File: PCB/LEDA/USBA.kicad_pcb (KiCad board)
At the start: 2 copper layers, 70 x 70 mm, 23 parts, among them J1 USB_A, J2 Conn_01x03, T1 T3902_MEMS_Mic, U2 ESP32-S3-MINI-1, U5 MD8942

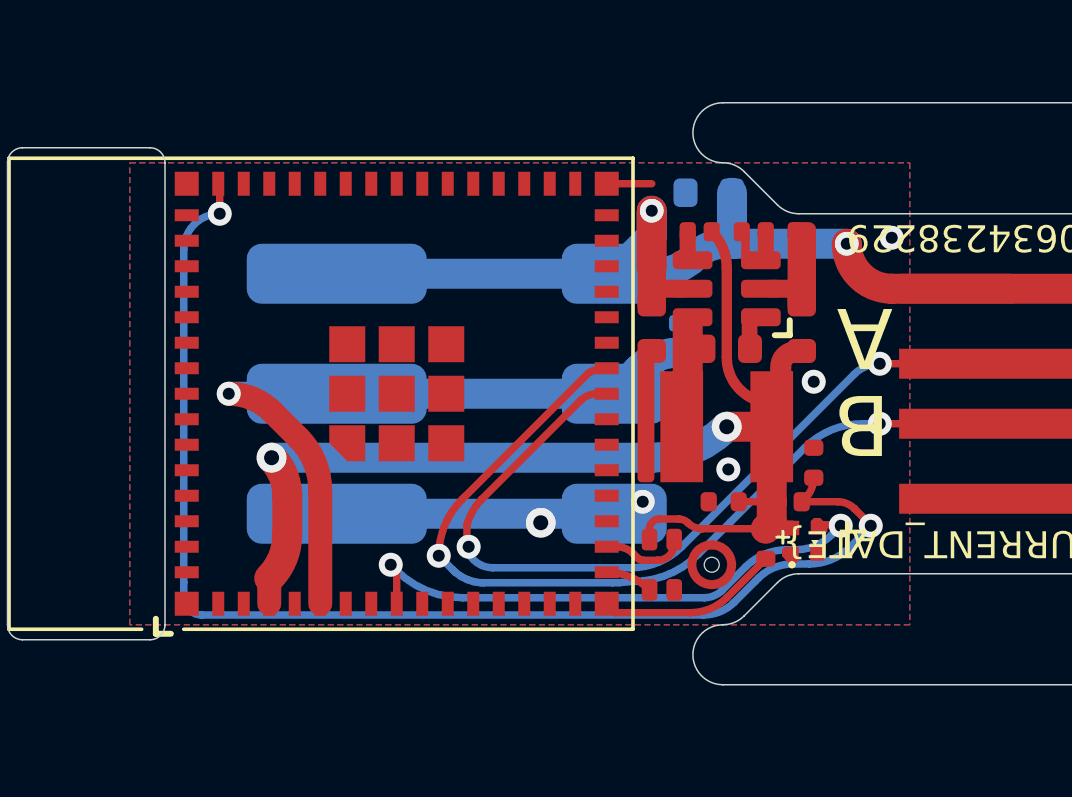
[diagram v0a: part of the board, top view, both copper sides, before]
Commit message: LEFT
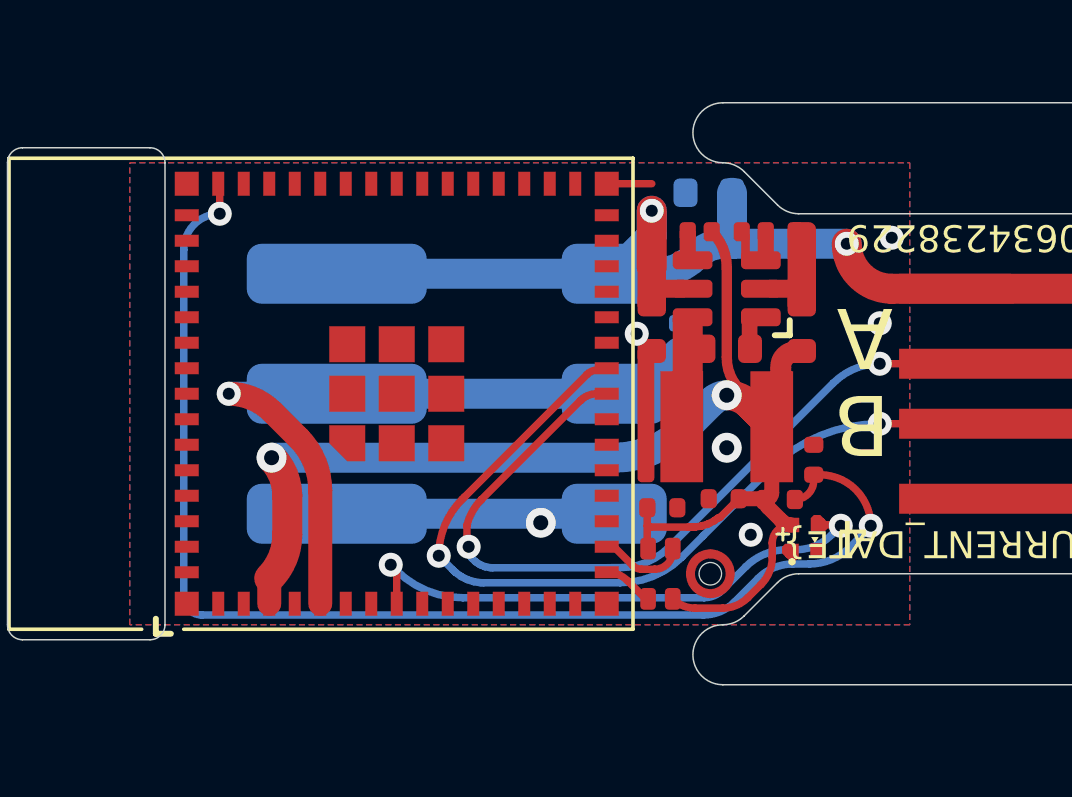
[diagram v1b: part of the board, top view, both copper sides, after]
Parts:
- moved C2 3.65 mm to (104.5, 103.1), turned to 0 degrees
- moved T1 0.30 mm to (105.3, 105.3)
- moved R1 0.24 mm to (108.4, 102.8)
- moved C1 0.10 mm to (106.5, 102.8)
- moved D1 0.10 mm to (109.2, 104.1)
- moved C3 0.10 mm to (109.5, 101.5)
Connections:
- T1 pad 2: GND -> +3.3V
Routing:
- net +3.3V: track 31.9 -> 39.0 mm
- net GND: track 16.8 -> 10.8 mm, vias 5 -> 6
- net VBUS: track 29.7 -> 28.5 mm
